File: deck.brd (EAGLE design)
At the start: 100 x 80 mm, 2 parts

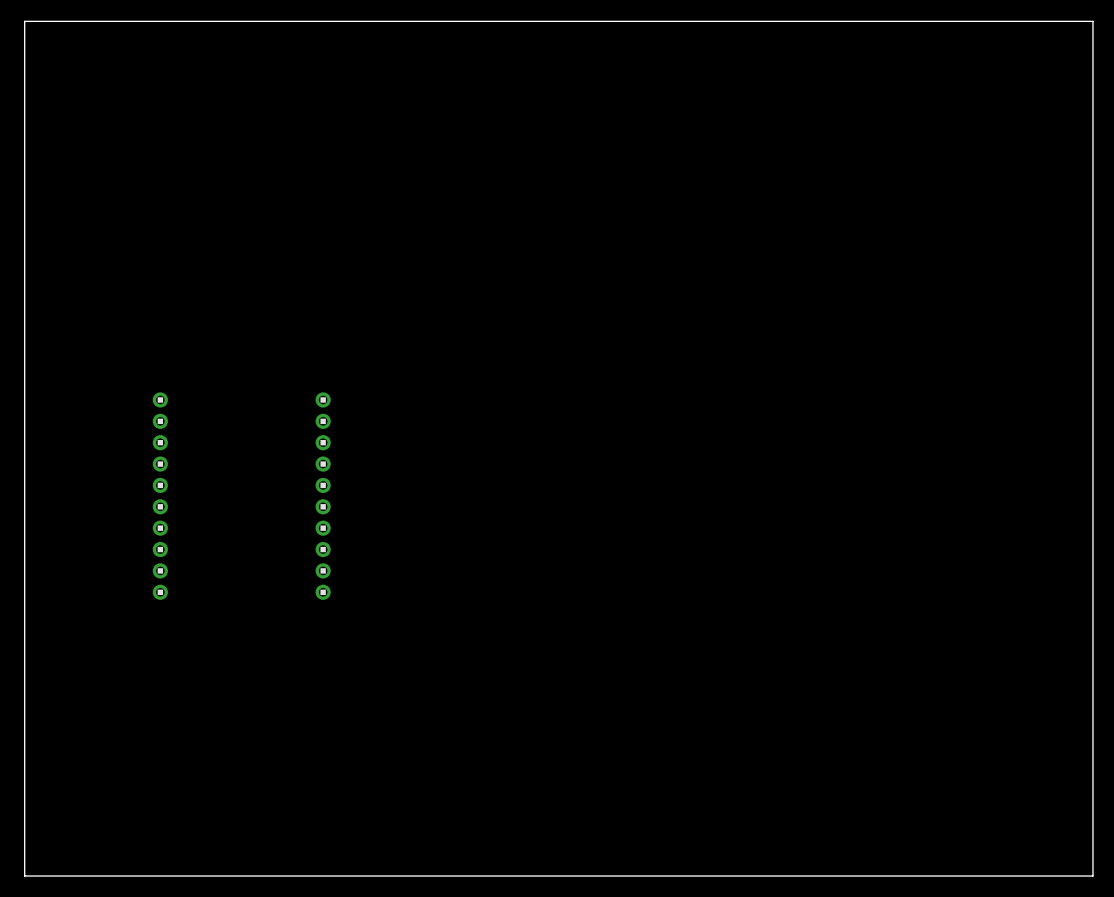
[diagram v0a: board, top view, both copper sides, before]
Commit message: More board design
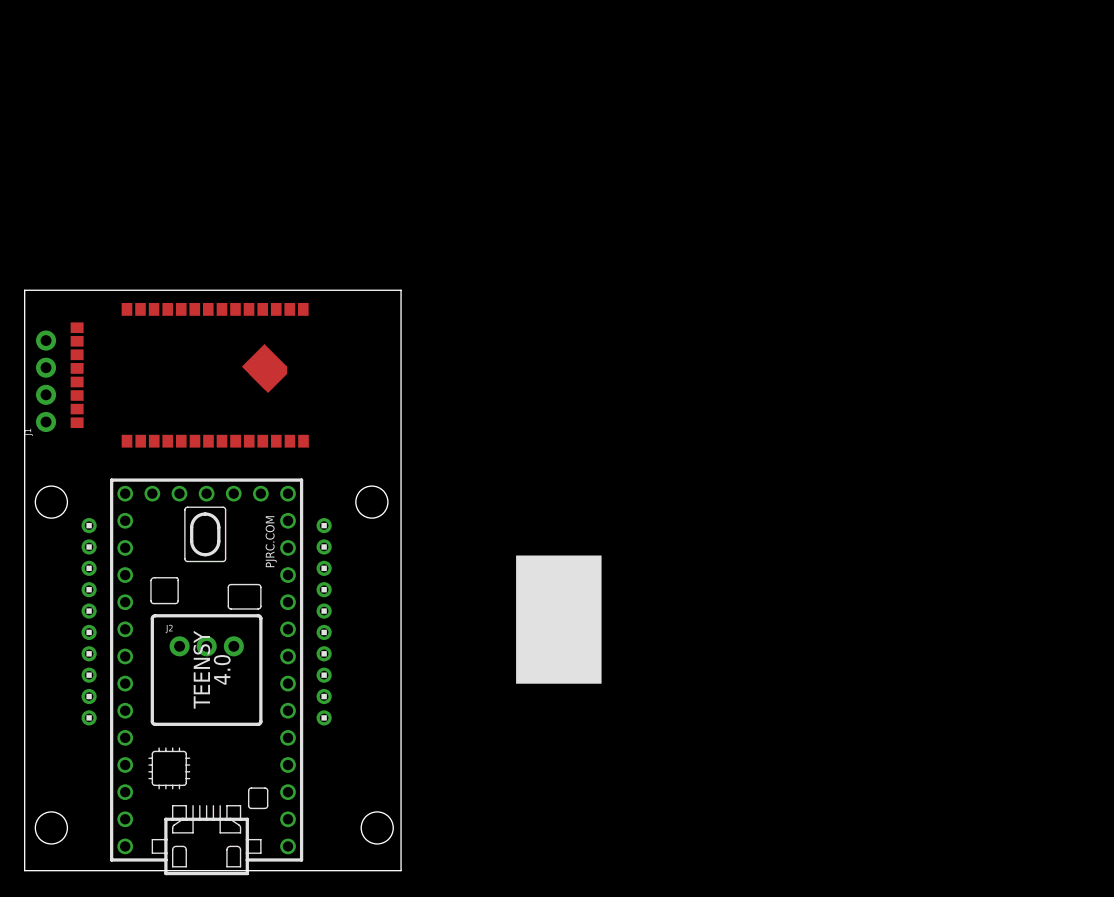
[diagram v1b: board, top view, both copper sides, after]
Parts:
- added J1: (no value), SparkFun-Connectors:1X04_NO_SILK
- added J2: (no value), SparkFun-Connectors:1X03_NO_SILK
- added U$3: TEENSY_4.0, TEENSY 4.0:TEENSY_4.0
- added U$4: TINYPICO-NANO-CONNECTOR, TinyPICO_NANO_Eagle:TINYPICO-NANO-CONNECTOR
- moved U$1 13.5 mm to (6.03, 23.8)
- moved U$2 11.8 mm to (28.0, 23.8)
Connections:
- new net 5V: U$4.5V
- new net VBAT: U$4.VBAT
- net 3V3: now also U$4.3V3
- net GND: now also U$4.GND$1, U$4.GND$2, U$4.GND$3, U$4.GND$4
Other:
- board size 100 x 80 mm -> 35.2 x 54.3 mm
